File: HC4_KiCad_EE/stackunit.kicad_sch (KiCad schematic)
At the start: 18 parts, among them IC11 74HC161, IC12 74HC377

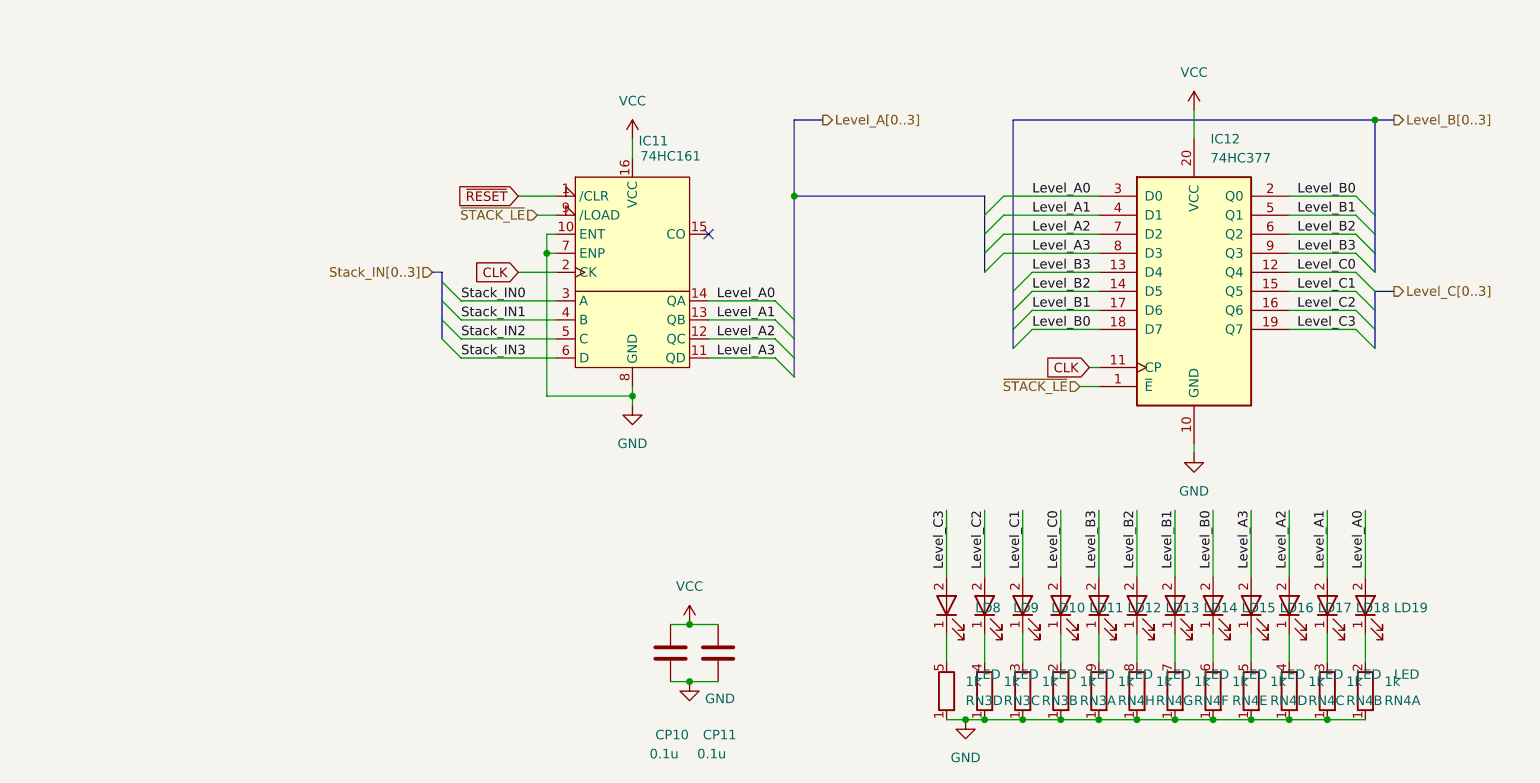
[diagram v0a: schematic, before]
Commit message: 一部を整地
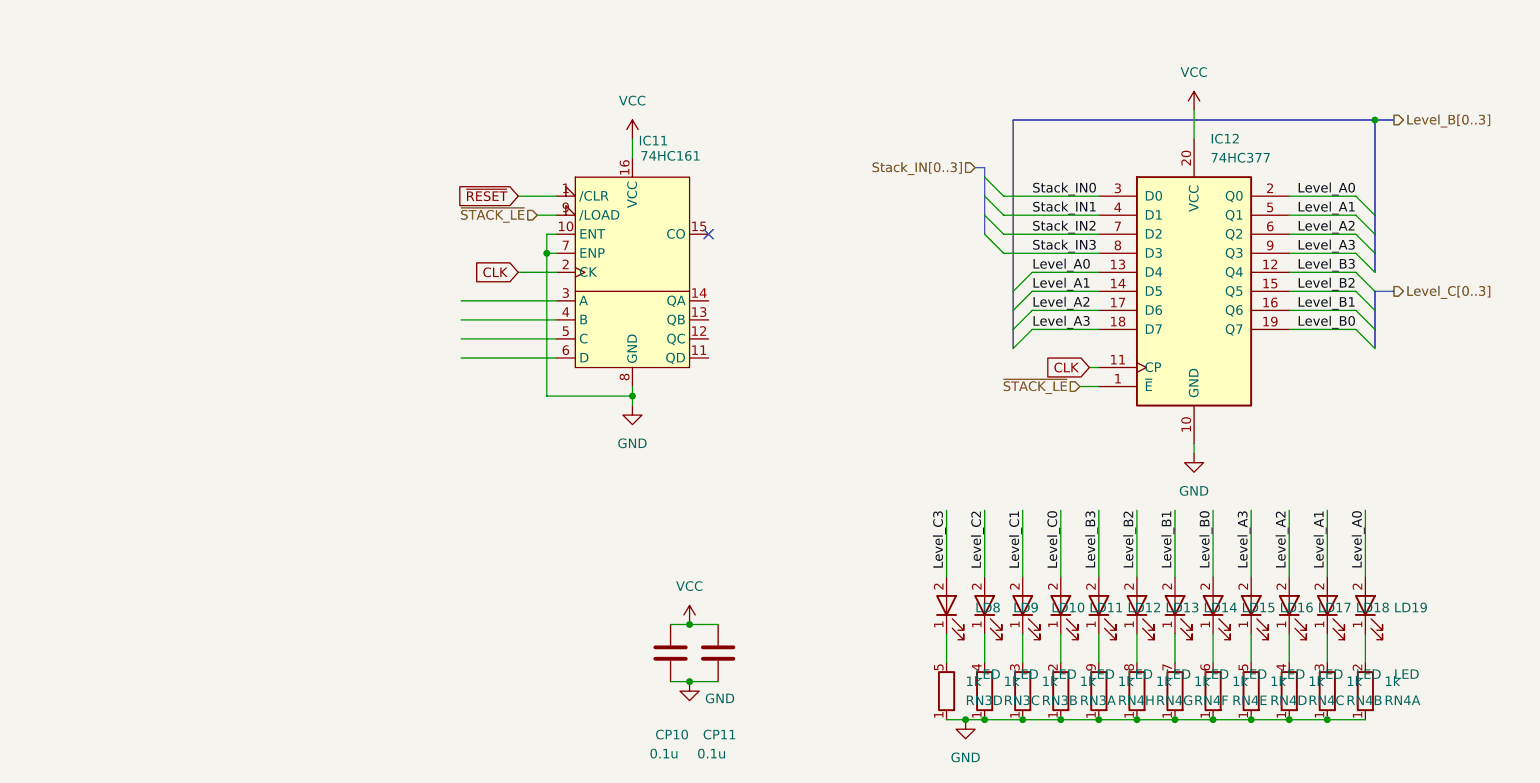
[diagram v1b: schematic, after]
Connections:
- net Level_A0: now also IC12.13 (D4), IC12.2 (Q0); no longer IC11.14 (QA), IC12.3 (D0)
- net Level_A1: now also IC12.14 (D5), IC12.5 (Q1); no longer IC11.13 (QB), IC12.4 (D1)
- net Level_A2: now also IC12.17 (D6), IC12.6 (Q2); no longer IC11.12 (QC), IC12.7 (D2)
- net Level_A3: now also IC12.18 (D7), IC12.9 (Q3); no longer IC11.11 (QD), IC12.8 (D3)
- net Level_B0: now also IC12.19 (Q7); no longer IC12.18 (D7), IC12.2 (Q0)
- net Level_B1: now also IC12.16 (Q6); no longer IC12.17 (D6), IC12.5 (Q1)
- net Level_B2: now also IC12.15 (Q5); no longer IC12.14 (D5), IC12.6 (Q2)
- net Level_B3: now also IC12.12 (Q4); no longer IC12.13 (D4), IC12.9 (Q3)
- net Level_C0: no longer IC12.12 (Q4)
- net Level_C1: no longer IC12.15 (Q5)
- net Level_C2: no longer IC12.16 (Q6)
- net Level_C3: no longer IC12.19 (Q7)
- net Stack_IN0: now also IC12.3 (D0); no longer IC11.3 (A)
- net Stack_IN1: now also IC12.4 (D1); no longer IC11.4 (B)
- net Stack_IN2: now also IC12.7 (D2); no longer IC11.5 (C)
- net Stack_IN3: now also IC12.8 (D3); no longer IC11.6 (D)

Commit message: コミット忘れてたてへ
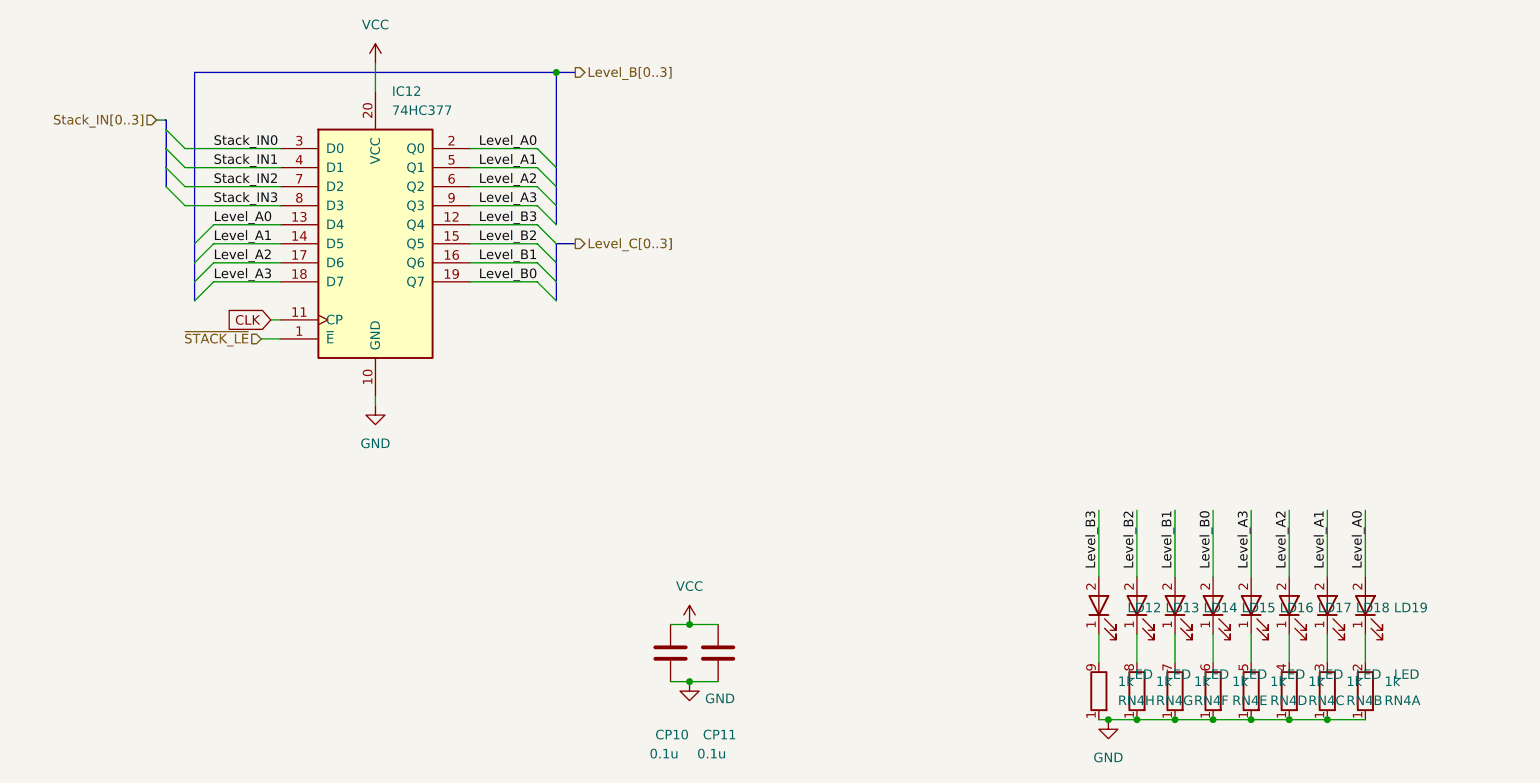
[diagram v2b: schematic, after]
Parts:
- removed IC11: 74HC161, Package_DIP:DIP-16_W7.62mm_Socket, symbol 74xx_2:74HC161
- removed LD10, LD11, LD8, LD9: LED, LED_THT:LED_Rectangular_W5.0mm_H2.0mm, symbol Device2:LED_
- removed RN3: 1k, Resistor_THT:R_Array_SIP5, symbol Device:R_Network04_Split
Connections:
- no-connect marks 1 -> 0
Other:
- moved on the sheet: IC12
